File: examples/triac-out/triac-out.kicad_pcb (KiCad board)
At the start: 2 copper layers, 43.2 x 21.6 mm, 11 parts, among them U1 MOC3021M

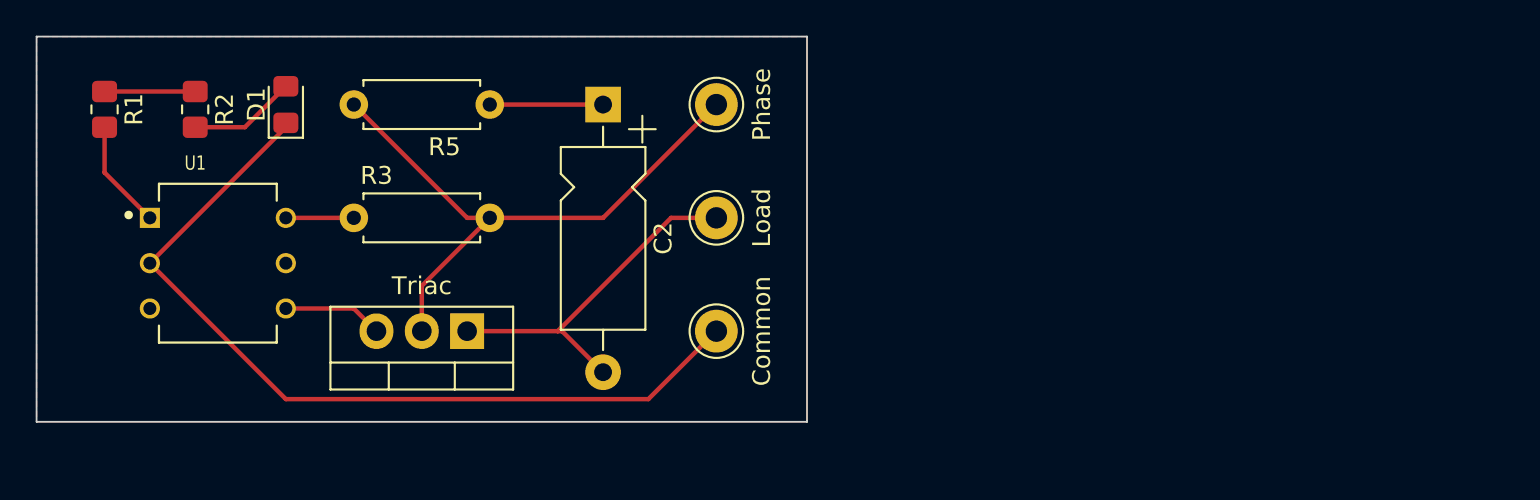
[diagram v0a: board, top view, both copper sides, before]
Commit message: Added examples.
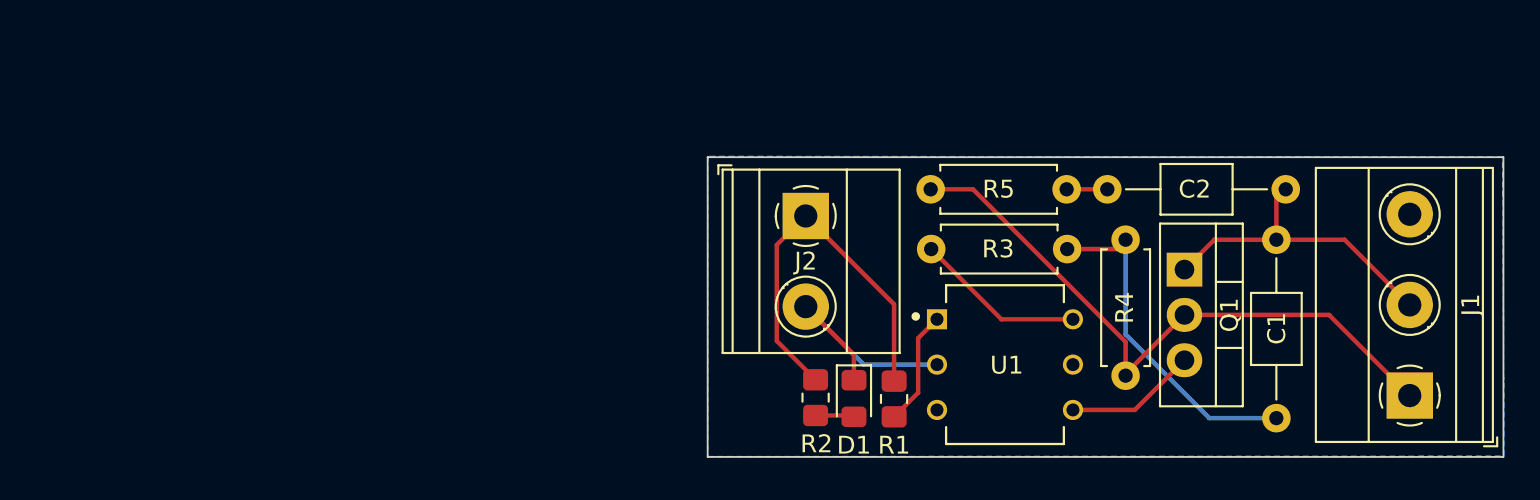
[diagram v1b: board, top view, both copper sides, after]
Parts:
- removed Common: Common, Connector_Pin:Pin_D1.0mm_L10.0mm_LooseFit
- removed Load: Load, Connector_Pin:Pin_D1.0mm_L10.0mm_LooseFit
- removed Phase: Phase, Connector_Pin:Pin_D1.0mm_L10.0mm_LooseFit
- removed Triac: BT136-600, Package_TO_SOT_THT:TO-220-3_Vertical
- added C1: 0nF, Capacitor_THT:C_Axial_L3.8mm_D2.6mm_P10.00mm_Horizontal, F.Cu at (167.3, 87.4)
- added J1: Power, TerminalBlock_Phoenix:TerminalBlock_Phoenix_MKDS-1,5-3-5.08_1x03_P5.08mm_Horizontal, F.Cu at (174.8, 86.2)
- added J2: DC_in, TerminalBlock_Phoenix:TerminalBlock_Phoenix_MKDS-1,5-2-5.08_1x02_P5.08mm_Horizontal, F.Cu at (140.9, 76.1)
- added Q1: Triac, Package_TO_SOT_THT:TO-220-3_Vertical, F.Cu at (162.1, 79.1)
- added R4: 470, Resistor_THT:R_Axial_DIN0207_L6.3mm_D2.5mm_P7.62mm_Horizontal, F.Cu at (158.8, 77.4)
- C2: footprint Capacitor_THT:CP_Axial_L10.0mm_D4.5mm_P15.00mm_Horizontal -> Capacitor_THT:C_Axial_L3.8mm_D2.6mm_P10.00mm_Horizontal
- R3: value 1k -> 330
- moved R1 47.1 mm to (145.8, 86.3)
- moved U1 44.5 mm to (152.1, 84.4)
- moved R2 38.3 mm to (141.4, 86.3)
- moved D1 35.8 mm to (143.6, 86.3), turned to -90 degrees
- moved R5 32.7 mm to (155.5, 74.6)
- moved R3 32.4 mm to (147.9, 78.0)
- moved C2 28.7 mm to (157.8, 74.6), turned to 0 degrees
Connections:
- net GND renamed GND1
- net Vin renamed /Vin
- R3 pad 2: Net_Phase -> Net-(C1-Pad1)
- R5 pad 2: Net_Phase -> /Phase
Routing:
- net /Phase: track 0.00 -> 35.6 mm
- net GND1: track 47.5 -> 13.9 mm
- net Net_Phase: track 33.5 -> 0.00 mm
- net Net-(C1-Pad1): track 0.00 -> 19.2 mm
- net /Vin: track 5.08 -> 22.2 mm
- net Net-(R3-Pad1): track 3.81 -> 9.57 mm
- net Net-(C2-Pad1): track 6.35 -> 2.28 mm
- net Net-(D1-A): track 6.03 -> 2.18 mm
- net /Load: track 20.1 -> 17.9 mm
- net /gate: track 5.61 -> 7.40 mm
- added copper zone on B.Cu, net (none)
- removed copper zone on F.Cu, net (none)
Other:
- board size 43.2 x 21.6 mm -> 44.6 x 16.8 mm
